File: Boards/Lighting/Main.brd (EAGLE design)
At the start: 56.8 x 36.8 mm, 49 parts, among them J1 AVR_SPI_PRG_6PTH

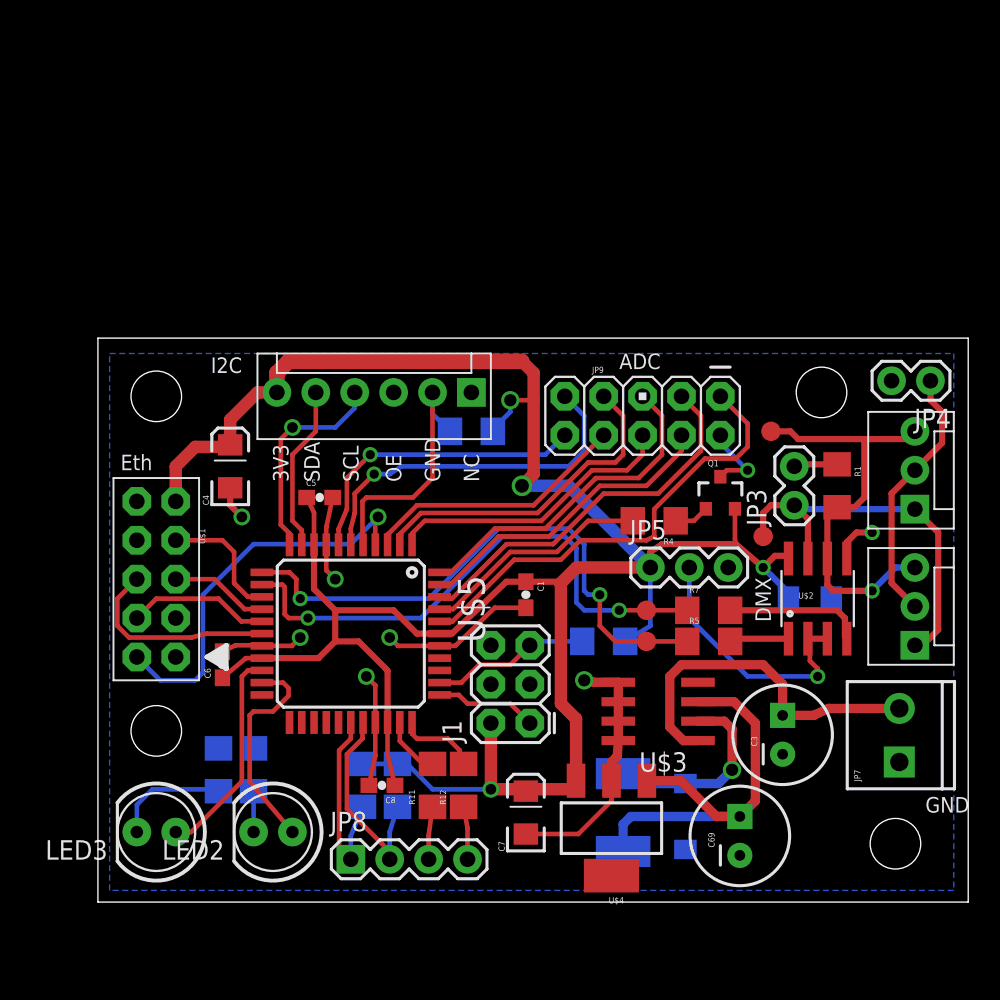
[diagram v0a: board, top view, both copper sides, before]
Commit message: Prepared board for production, last minute error checks and rotations
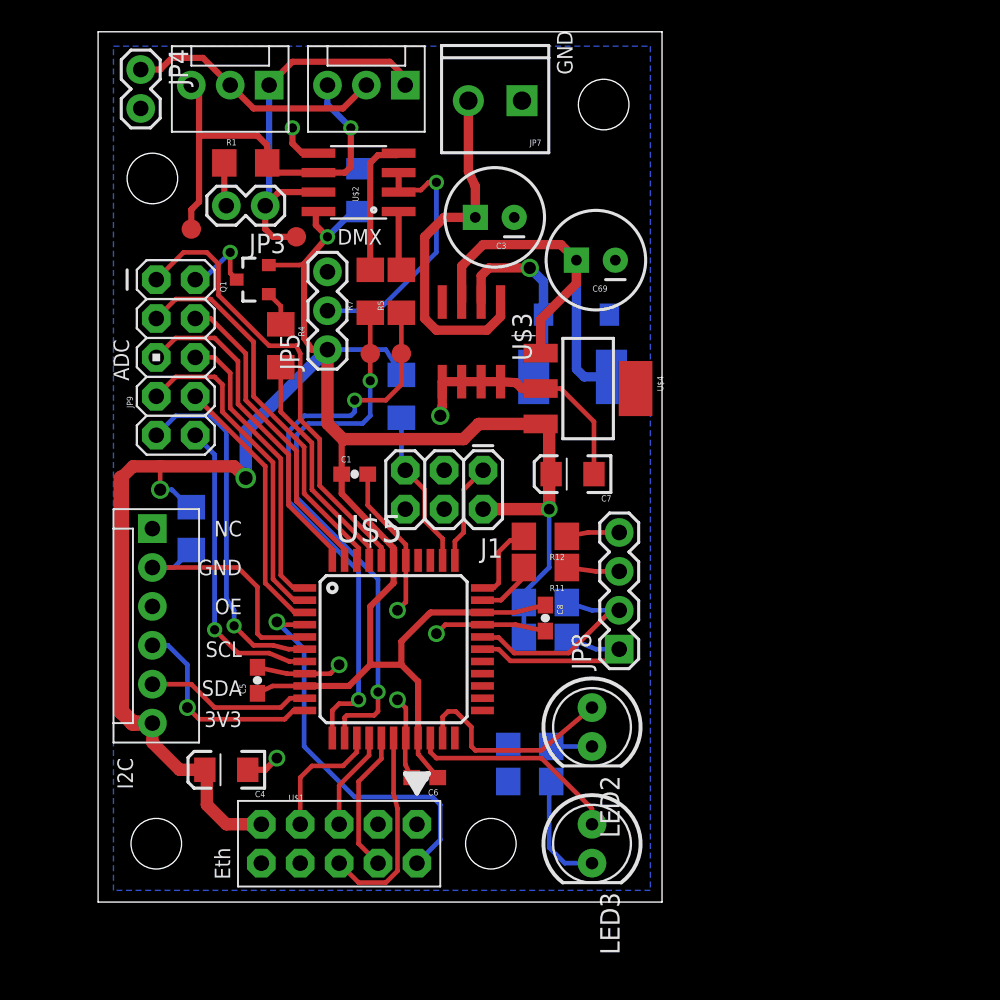
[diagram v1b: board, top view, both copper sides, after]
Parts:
- moved JP4 55.4 mm to (2.79, 54.4), turned to 270 degrees
- moved STANDOFF4 51.9 mm to (33.0, 52.1), turned to 90 degrees
- moved JP1 50.4 mm to (11.2, 53.3), turned to 180 degrees
- moved JP7 49.7 mm to (27.7, 52.3), turned to 180 degrees
- moved JP2 49.4 mm to (20.1, 53.3), turned to 180 degrees
- moved STANDOFF3 45.9 mm to (3.56, 47.2), turned to 90 degrees
- moved R1 44.0 mm to (9.65, 48.3), turned to 0 degrees
- moved U$2 40.5 mm to (17.0, 47.0), turned to 90 degrees
- moved TP4 40.1 mm to (6.10, 43.9), turned to 90 degrees
- moved C2 39.7 mm to (17.0, 46.5), turned to 270 degrees
- moved JP3 39.7 mm to (10.9, 45.5), turned to 180 degrees
- moved C69 38.7 mm to (32.5, 41.9), turned to 180 degrees
- moved C3 38.7 mm to (25.9, 44.7), turned to 180 degrees
- moved TP3 36.2 mm to (13.0, 43.4), turned to 90 degrees
- moved Q1 33.5 mm to (10.2, 40.6), turned to 90 degrees
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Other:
- board size 56.8 x 36.8 mm -> 36.8 x 56.8 mm
